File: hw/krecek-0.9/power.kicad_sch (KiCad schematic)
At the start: 1 part, among them U3 BQ24045DSQR

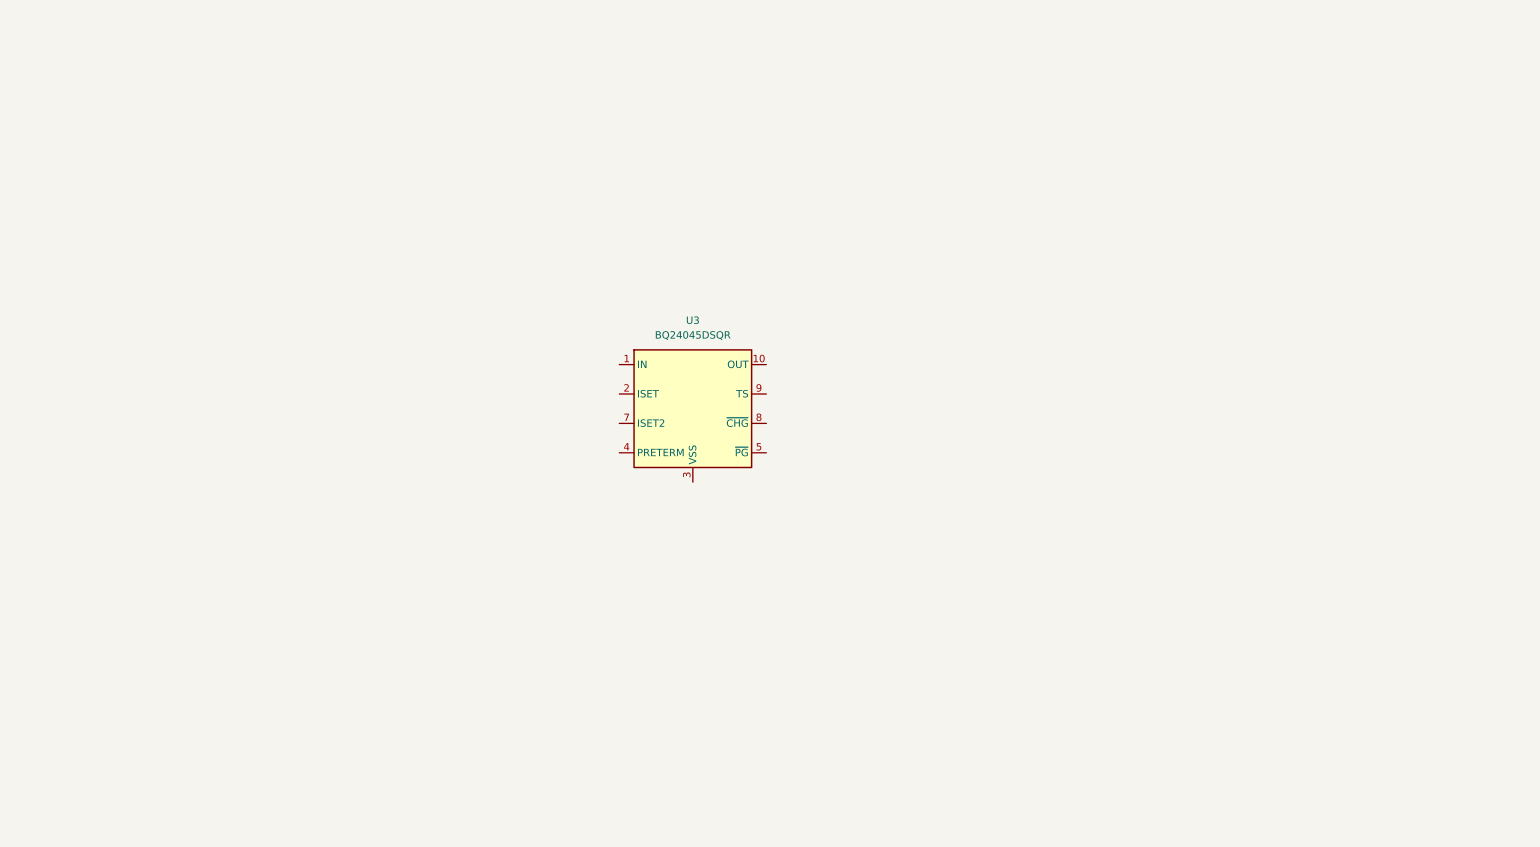
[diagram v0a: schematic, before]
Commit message: More work on power supply section
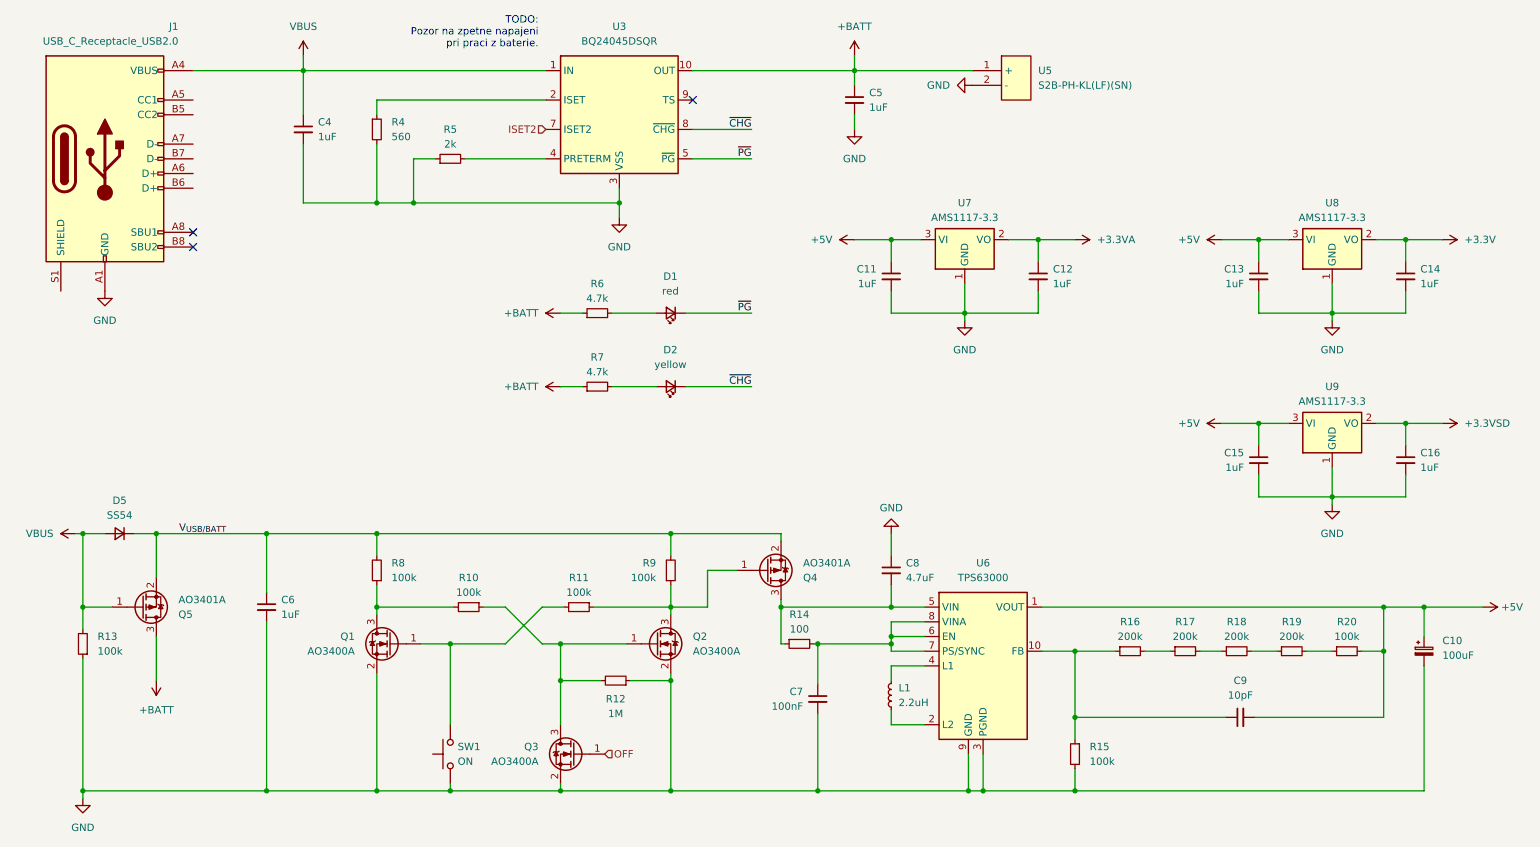
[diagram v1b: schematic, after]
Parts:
- added C10: 100uF, Capacitor_Tantalum_SMD:CP_EIA-3528-21_Kemet-B, symbol Device:C_Polarized_Small
- added C11, C12, C13, C14, C15, C16, C4, C5, C6: 1uF, Capacitor_SMD:C_0805_2012Metric, symbol Device:C_Small
- added C7: 100nF, Capacitor_SMD:C_0402_1005Metric, symbol Device:C_Small
- added C8: 4.7uF, Capacitor_SMD:C_0603_1608Metric, symbol Device:C_Small
- added C9: 10pF, Capacitor_SMD:C_0402_1005Metric, symbol Device:C_Small
- added D1: red, LED_SMD:LED_0603_1608Metric, symbol Device:LED_Small
- added D2: yellow, LED_SMD:LED_0603_1608Metric, symbol Device:LED_Small
- added D5: SS54, Diode_SMD:D_SMA, symbol Device:D_Small
- added J1: USB_C_Receptacle_USB2.0, LCSC:USB-C-SMD_TYPEC-304J-BCP16, symbol Connector:USB_C_Receptacle_USB2.0
- added L1: 2.2uH, Inductor_SMD:L_1008_2520Metric, symbol Device:L_Small
- added Q1, Q2, Q3: AO3400A, Package_TO_SOT_SMD:SOT-23, symbol Transistor_FET:AO3400A
- added Q4, Q5: AO3401A, Package_TO_SOT_SMD:SOT-23, symbol Transistor_FET:AO3401A
- added R10, R11, R13, R15, R20, R8, R9: 100k, Resistor_SMD:R_0402_1005Metric, symbol Device:R_Small
- added R12: 1M, Resistor_SMD:R_0402_1005Metric, symbol Device:R_Small
- added R14: 100, Resistor_SMD:R_0402_1005Metric, symbol Device:R_Small
- added R16, R17, R18, R19: 200k, Resistor_SMD:R_0402_1005Metric, symbol Device:R_Small
- added R4: 560, Resistor_SMD:R_0603_1608Metric, symbol Device:R_Small
- added R5: 2k, Resistor_SMD:R_0402_1005Metric, symbol Device:R_Small
- added R6, R7: 4.7k, Resistor_SMD:R_0402_1005Metric, symbol Device:R_Small
- added SW1: ON, symbol Switch:SW_Push
- added U5: S2B-PH-KL(LF)(SN), LCSC:CONN-TH-2P-P2.00_S2B-PH-KL-LF-SN, symbol LCSC:S2B-PH-KL(LF)(SN)
- added U6: TPS63000, Package_SON:Texas_DRC0010J_ThermalVias, symbol Regulator_Switching:TPS63000
- added U7, U8, U9: AMS1117-3.3, Package_TO_SOT_SMD:SOT-223-3_TabPin2, symbol Regulator_Linear:AMS1117-3.3
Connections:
- net VBUS: now reaches U3.1 (IN)
- net VBUS: now also C4.1, D5.2 (A), J1.A4 (VBUS), J1.A9 (VBUS), J1.B4 (VBUS), J1.B9 (VBUS), Q5.1 (G), R13.2
- net +BATT: now reaches U3.10 (OUT)
- net +BATT: now also C5.1, Q5.3 (D), R6.1, R7.1, U5.1 (+)
- net GND: now reaches U3.11 (VSS), U3.3 (VSS)
- net GND: now also C10.2, C11.2, C12.2, C13.2, C14.2, C15.2, C16.2, C4.2, C5.2, C6.2, C7.2, C8.1, J1.A1 (GND), J1.A12 (GND), J1.B1 (GND), J1.B12 (GND), Q1.2 (S), Q2.2 (S), Q3.2 (S), R12.1, R13.1, R15.2, R4.2, R5.1, SW1.1, U5.2 (-), U6.11 (PGND), U6.3 (PGND), U6.9 (GND), U7.1 (GND), U8.1 (GND), U9.1 (GND)
- net at U3.2 (ISET): now also R4.1
- net at U3.4 (PRETERM): now also R5.2
- net ~{PG}: now reaches U3.5 (~{PG})
- net ~{PG}: now also D1.1 (K)
- net ISET2: now reaches U3.7 (ISET2)
- net ~{CHG}: now reaches U3.8 (~{CHG})
- net ~{CHG}: now also D2.1 (K)
- new net: C9.1, R15.1, R16.1, U6.10 (FB)
- new net: Q1.1 (G), R11.2, SW1.2
- new net: R18.2, R19.1
- new net: R19.2, R20.1
- new net: L1.1, U6.2 (L2)
- new net: L1.2, U6.4 (L1)
- new net: Q2.1 (G), Q3.3 (D), R10.1, R12.2
- new net: Q1.3 (D), R10.2, R8.1
- new net: C8.2, Q4.3 (D), R14.1, U6.5 (VIN)
- new net: C7.1, R14.2, U6.6 (EN), U6.7 (PS/SYNC), U6.8 (VINA)
- new net: Q2.3 (D), Q4.1 (G), R11.1, R9.1
- new net: D2.2 (A), R7.2
- new net: R17.2, R18.1
- new net: R16.2, R17.1
- new net: D1.2 (A), R6.2
- new net +3.3V: C14.1, U8.2 (VO)
- new net +3.3VA: C12.1, U7.2 (VO)
- new net +3.3VSD: C16.1, U9.2 (VO)
- new net +5V: C10.1, C11.1, C13.1, C15.1, C9.2, R20.2, U6.1 (VOUT), U7.3 (VI), U8.3 (VI), U9.3 (VI)
- new net OFF: Q3.1 (G)
- new net V_{USB/BATT}: C6.1, D5.1 (K), Q4.2 (S), Q5.2 (S), R8.2, R9.2
- no-connect marks 0 -> 3
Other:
- note added: "TODO: Pozor na zpetne napajeni pri praci z baterie."
- moved on the sheet: U3
